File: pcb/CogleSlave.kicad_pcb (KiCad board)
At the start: 2 copper layers, 24.9 x 20.8 mm, 7 parts, among them P1 CONN_01X04, P2 CONN_01X04, P3 CONN_01X08, U1 PCF8591T

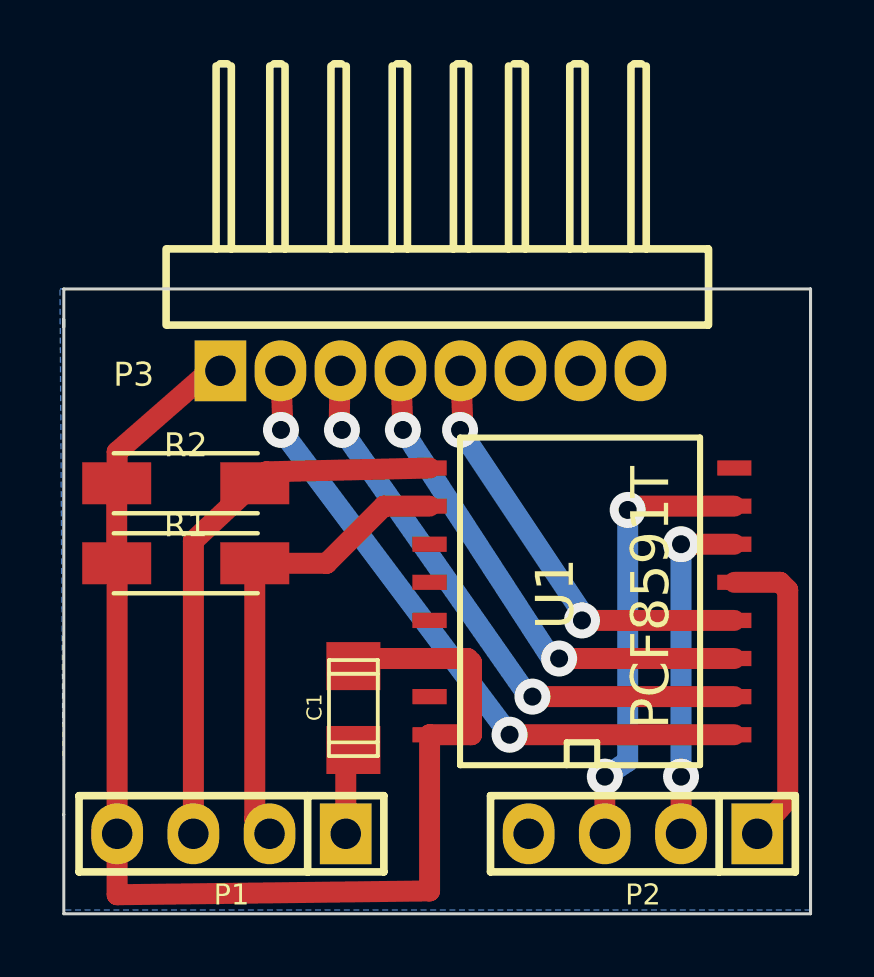
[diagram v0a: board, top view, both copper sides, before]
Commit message: 基板レイアウトを修正 1.2
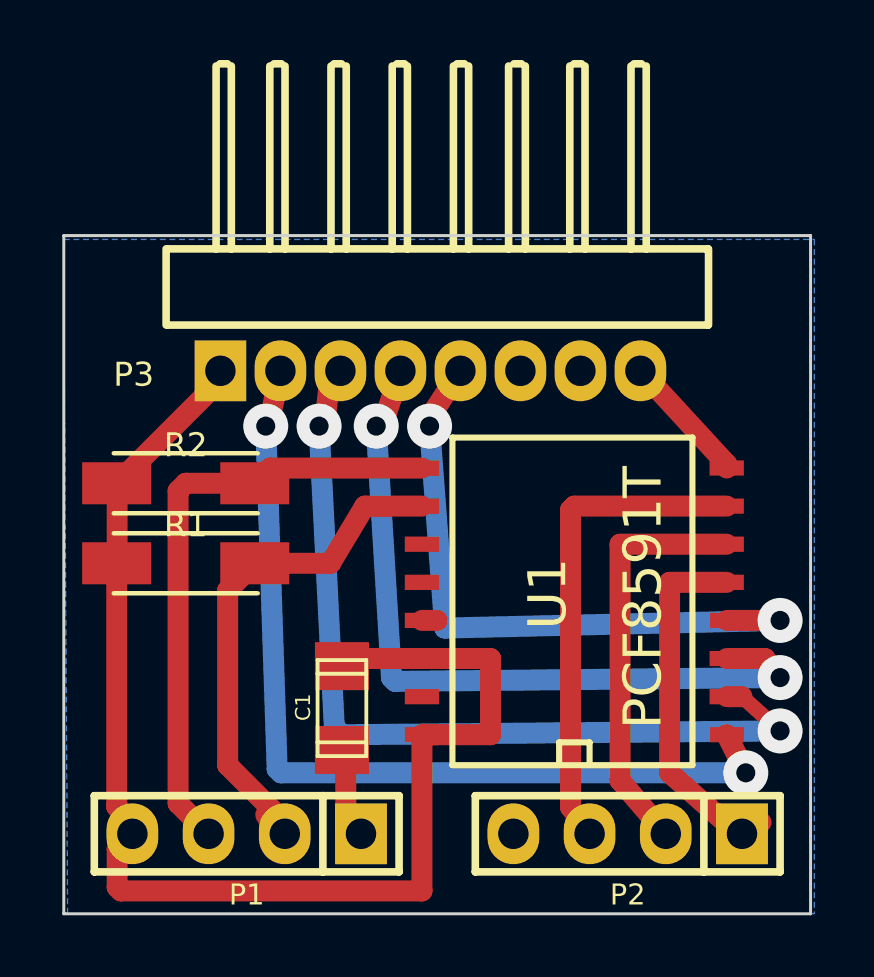
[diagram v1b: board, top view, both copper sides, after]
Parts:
- moved P1 0.51 mm to (176.8, 118.7)
- moved P2 0.51 mm to (189.5, 118.7)
- moved C1 0.38 mm to (180.0, 114.6)
- moved U1 0.25 mm to (187.7, 111.0)
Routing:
- net /AIN1: track 20.0 -> 29.1 mm
- net /AIN2: track 17.5 -> 25.5 mm
- net /AIN0: track 22.5 -> 30.5 mm
- net /AIN3: track 15.0 -> 21.9 mm
- net GND: track 2.90 -> 7.97 mm
- net /A1: track 11.4 -> 13.8 mm, vias 2 -> 0
- net +5V: track 42.9 -> 45.0 mm
- net /SDA: track 18.6 -> 20.6 mm
- net /SCL: track 15.8 -> 17.8 mm
- net /A0: track 10.4 -> 12.0 mm
- net /A2: track 14.8 -> 16.3 mm, vias 2 -> 0
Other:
- board size 24.9 x 20.8 mm -> 24.9 x 22.6 mm
- net class Default: via_dia 1.2 -> 1.5
- rule via_min_size: 1.2 -> 1.3
